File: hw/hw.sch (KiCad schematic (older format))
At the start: 23 parts, among them J1 Motor 1 Connector, J2 Motor 2 Connector, J3 Distance sensor 3, J4 Distance sensor 1, J5 Distance sensor 2, J6 Distance sensor 6, J7 Distance sensor 4, J8 Distance sensor 5, U1 TB6612FNG_Breakout

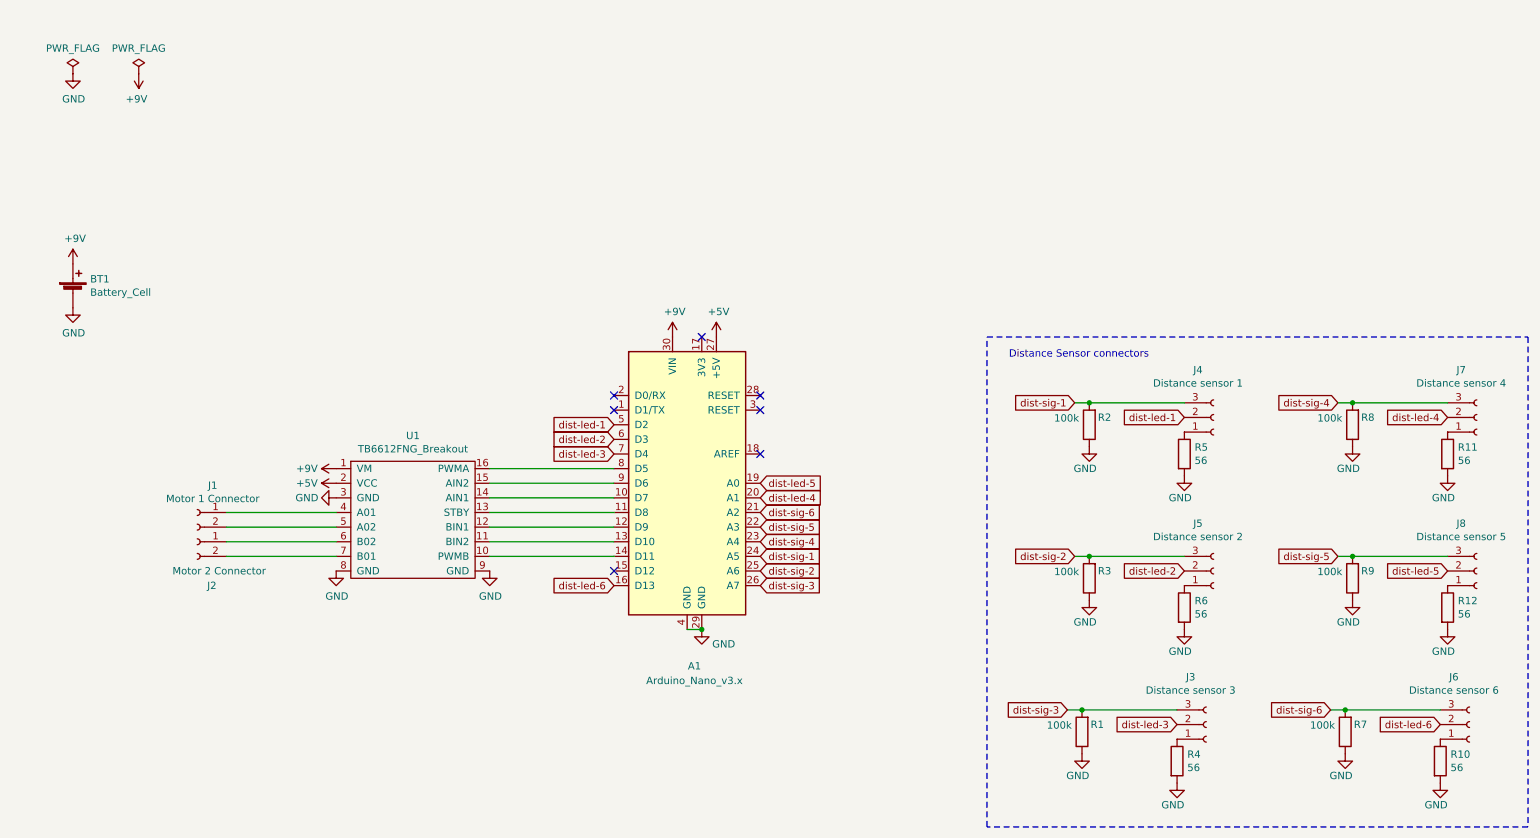
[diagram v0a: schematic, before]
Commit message: new pcb version
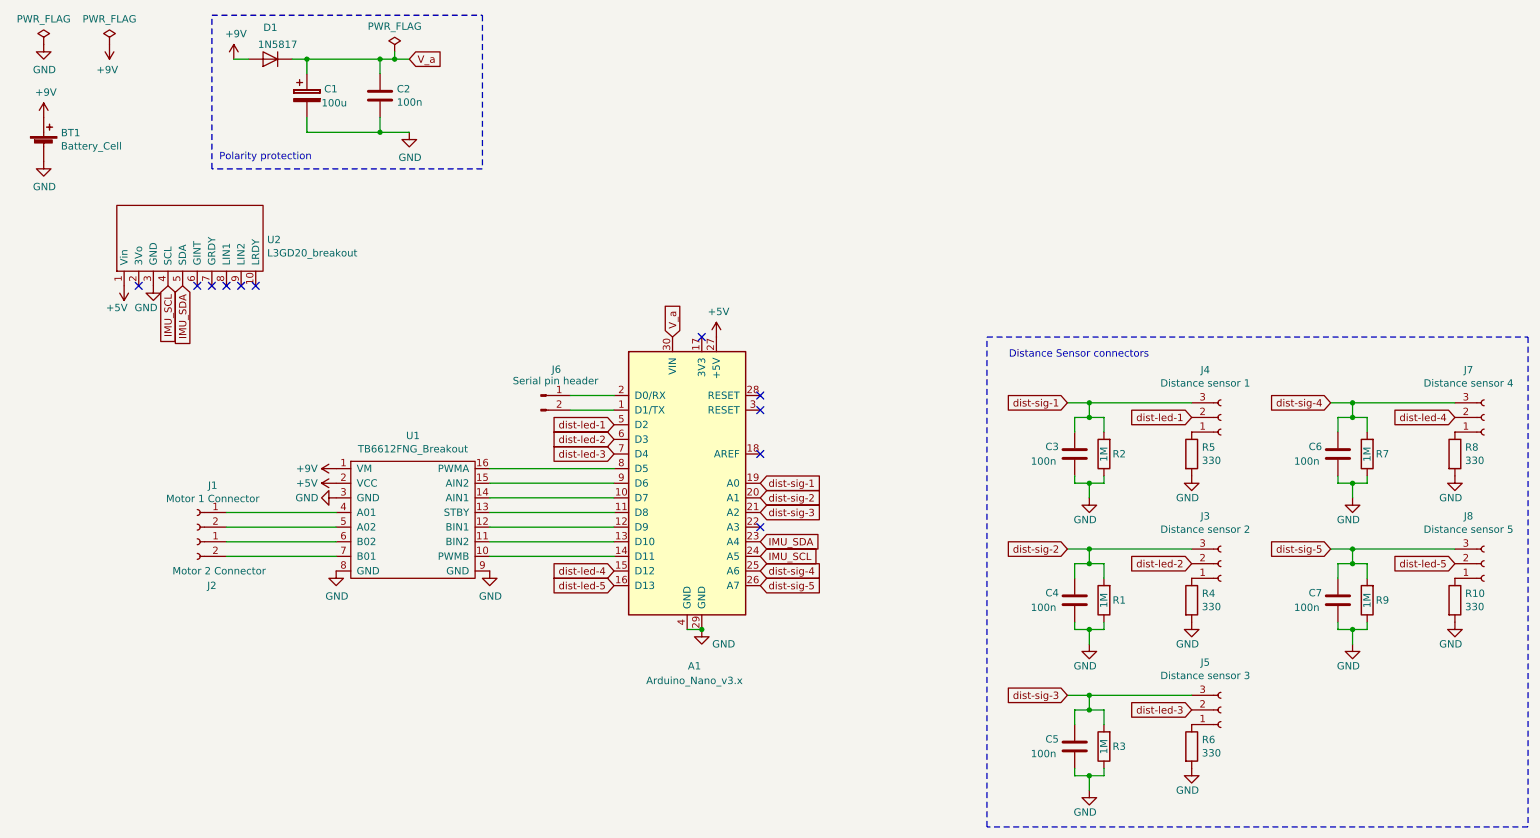
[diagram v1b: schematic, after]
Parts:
- removed J6: Distance sensor 6, Connector_PinSocket_2.54mm:PinSocket_1x03_P2.54mm_Vertical, symbol Connector:Conn_01x03_Female
- removed R11, R12: 56, Resistor_THT:R_Axial_DIN0207_L6.3mm_D2.5mm_P7.62mm_Horizontal, symbol Device:R
- added C1: 100u, Capacitor_THT:CP_Radial_D6.3mm_P2.50mm, symbol Device:CP
- added C2, C3, C4, C5, C6, C7: 100n, Capacitor_SMD:C_0805_2012Metric_Pad1.15x1.40mm_HandSolder, symbol Device:C
- added D1: 1N5817, Diode_THT:D_DO-41_SOD81_P7.62mm_Horizontal, symbol Device:D
- added J6: Serial pin header, Connector_PinHeader_2.54mm:PinHeader_1x02_P2.54mm_Vertical, symbol Connector:Conn_01x02_Male
- added U2: L3GD20_breakout, custom:L3GD20_breakout, symbol custom:L3GD20_breakout
- J3: value Distance sensor 3 -> Distance sensor 2
- J5: value Distance sensor 2 -> Distance sensor 3
- R1, R2, R3, R7, R9: value 100k -> 1M; footprint Resistor_THT:R_Axial_DIN0207_L6.3mm_D2.5mm_P7.62mm_Horizontal -> Resistor_SMD:R_0805_2012Metric_Pad1.15x1.40mm_HandSolder
- R10, R4, R5, R6: value 56 -> 330; footprint Resistor_THT:R_Axial_DIN0207_L6.3mm_D2.5mm_P7.62mm_Horizontal -> Resistor_SMD:R_0805_2012Metric_Pad1.15x1.40mm_HandSolder
- R8: value 100k -> 330; footprint Resistor_THT:R_Axial_DIN0207_L6.3mm_D2.5mm_P7.62mm_Horizontal -> Resistor_SMD:R_0805_2012Metric_Pad1.15x1.40mm_HandSolder
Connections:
- net dist-led-6 is gone; now on net dist-led-5: A1.16 (D13)
- net +5V: now also U2.1 (Vin)
- net +9V: now also D1.2 (A); no longer A1.30 (VIN)
- net GND: now also R8.2, C1.2, C2.2, C3.2, C4.2, C5.2, C6.2, C7.2, U2.3 (GND); no longer R8.1
- net dist-led-2: now also J3.2 (Pin_2); no longer J5.2 (Pin_2)
- net dist-led-3: now also J5.2 (Pin_2); no longer J3.2 (Pin_2)
- net dist-led-4: now also A1.15 (D12); no longer A1.20 (A1)
- net dist-led-5: no longer A1.19 (A0)
- net dist-sig-1: now also A1.19 (A0), C3.1; no longer A1.24 (A5)
- net dist-sig-2: now also A1.20 (A1), J3.3 (Pin_3), R1.2, C4.1; no longer A1.25 (A6), J5.3 (Pin_3), R3.2
- net dist-sig-3: now also A1.21 (A2), J5.3 (Pin_3), R3.2, C5.1; no longer A1.26 (A7), J3.3 (Pin_3), R1.2
- net dist-sig-4: now also A1.25 (A6), R7.2, C6.1; no longer A1.23 (A4), R8.2
- net dist-sig-5: now also A1.26 (A7), C7.1; no longer A1.22 (A3)
- net at A1.1 (D1/TX): now also J6.2 (Pin_2)
- net at A1.2 (D0/RX): now also J6.1 (Pin_1)
- net at J7.1 (Pin_1): now also R8.1
- net at J8.1 (Pin_1): now also R10.1
- removed net dist-sig-6: A1.21 (A2), R7.2
- new net IMU_SCL: A1.24 (A5), U2.4 (SCL)
- new net IMU_SDA: A1.23 (A4), U2.5 (SDA)
- new net V_a: A1.30 (VIN), C1.1, C2.1, D1.1 (K)
- no-connect marks 7 -> 11
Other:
- note added: "Polarity protection"
- moved on the sheet: BT1, J4, R2, R5
